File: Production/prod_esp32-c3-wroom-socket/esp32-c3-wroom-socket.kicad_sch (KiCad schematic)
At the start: 15 parts, among them J1 USB-C_Receptacle_Data_16P_GCT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, J3 USB-C_KUSBX-SL-CS1N14-B, SW2 SW_Push_SMD_6x3.5, U1 ESP32-C3-WROOM-02-N4, U2 AMS1117-3V3

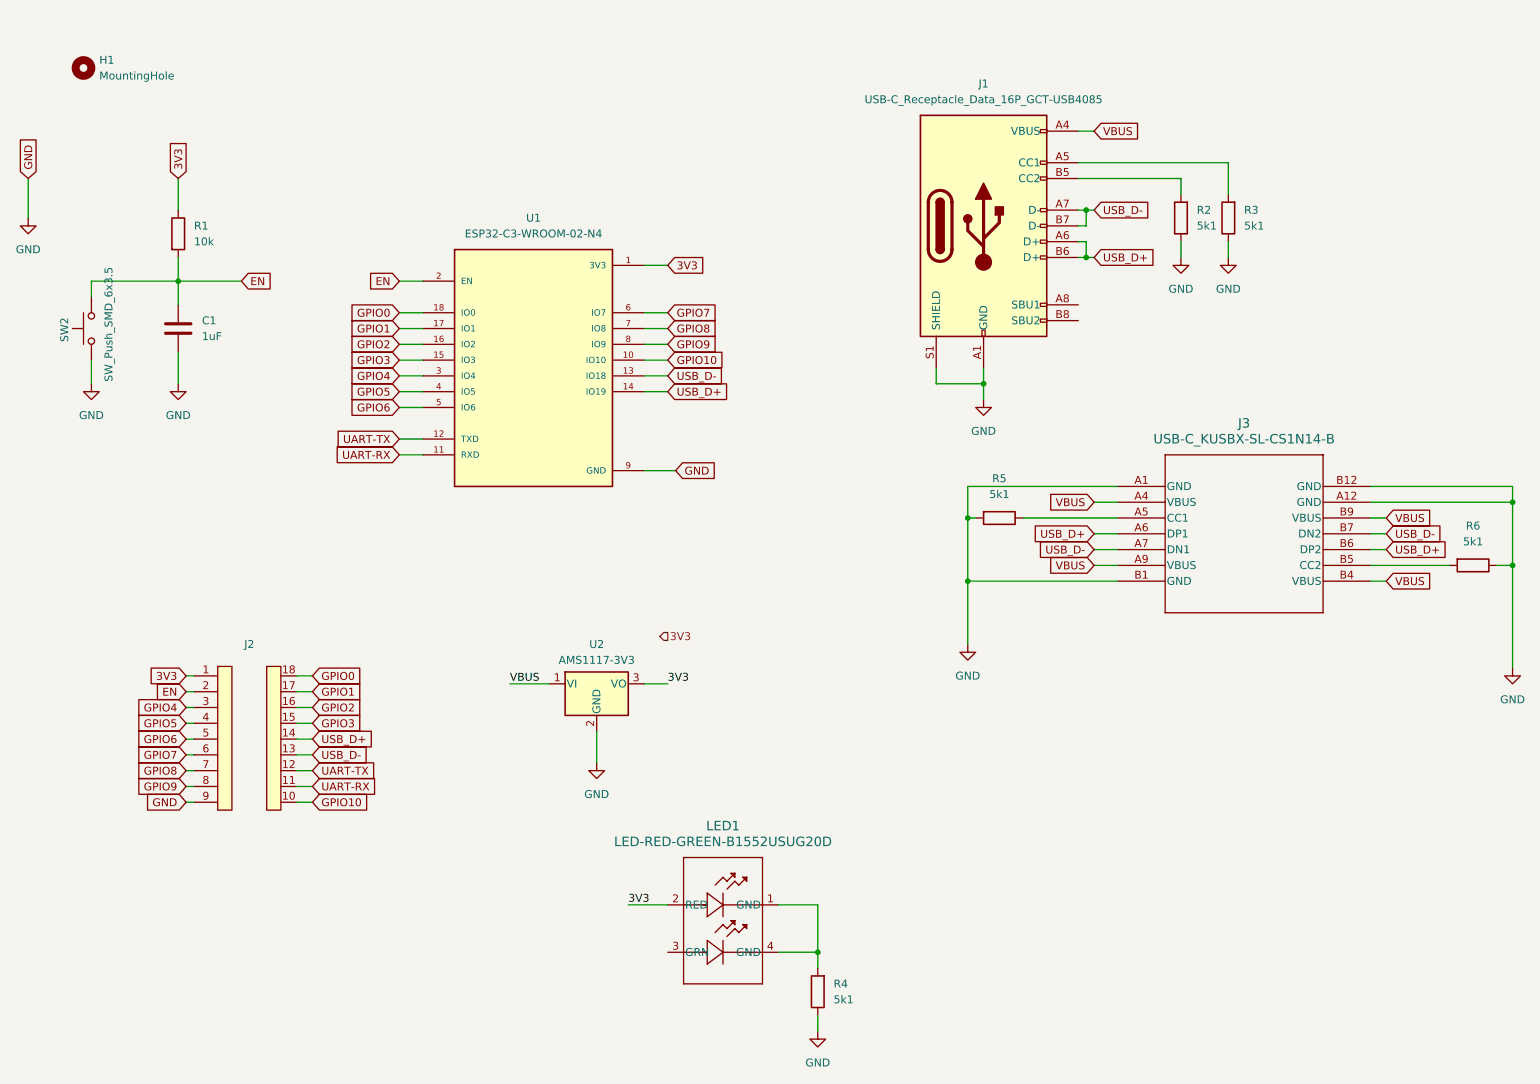
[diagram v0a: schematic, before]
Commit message: .
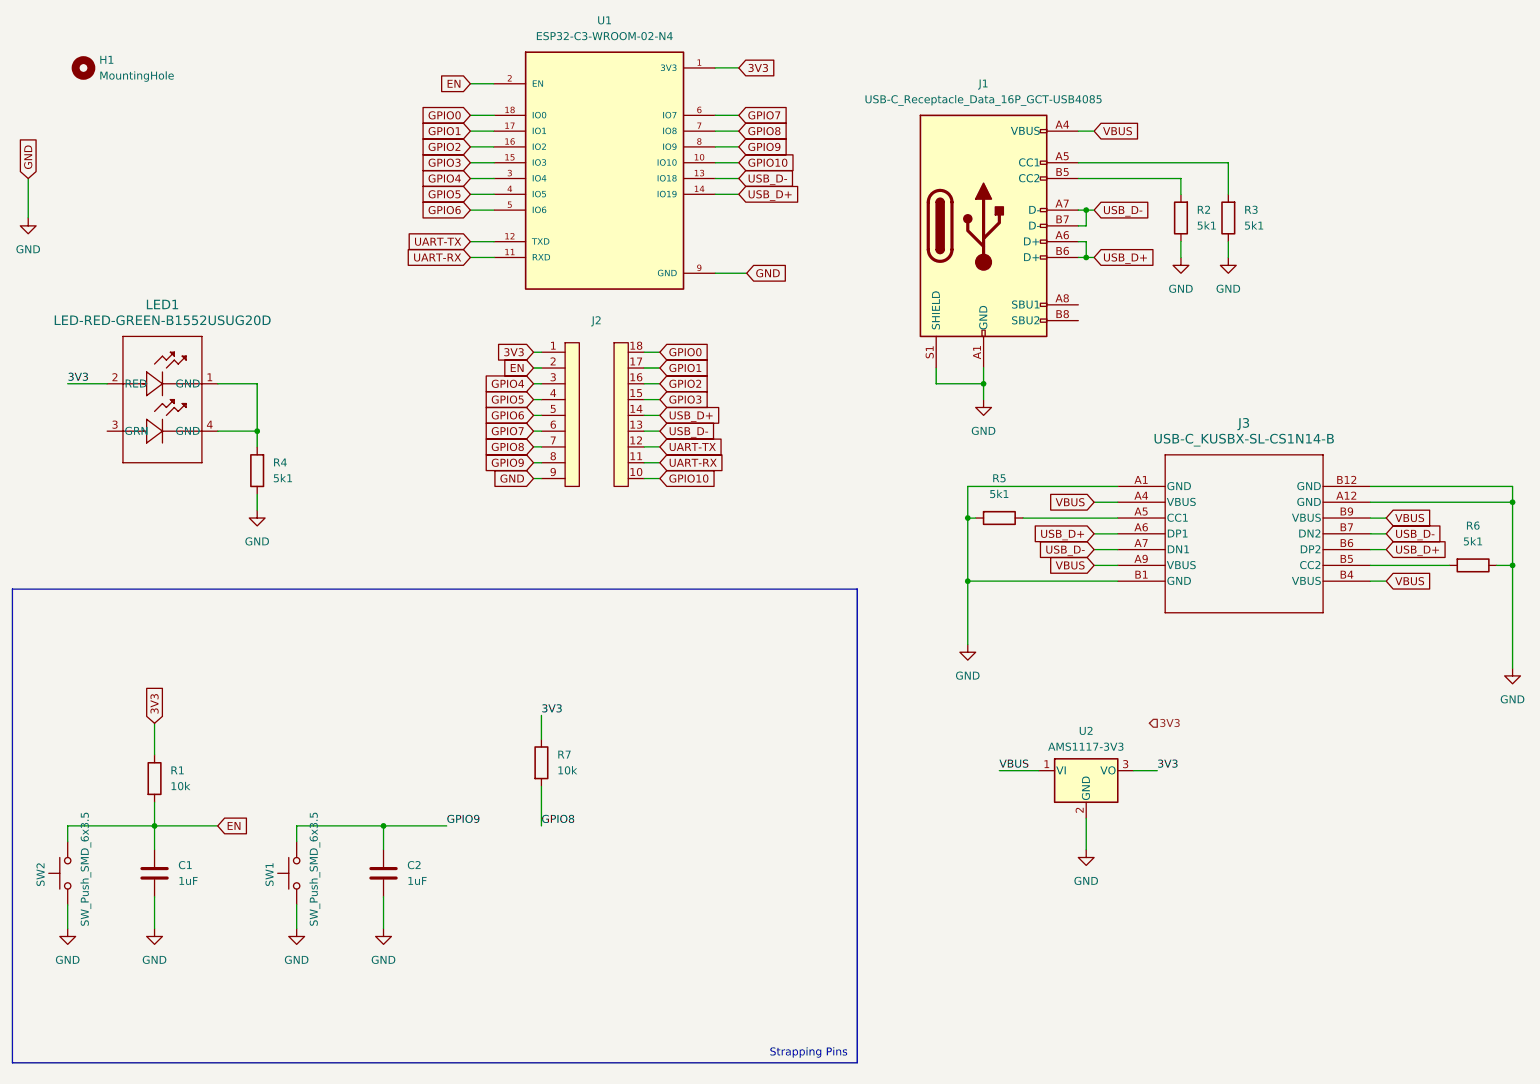
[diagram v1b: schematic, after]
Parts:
- added C2: 1uF, Resistor_SMD:R_0612_1632Metric_Pad1.18x3.40mm_HandSolder, symbol Device:C
- added R7: 10k, Resistor_SMD:R_1206_3216Metric_Pad1.30x1.75mm_HandSolder, symbol Device:R
- added SW1: SW_Push_SMD_6x3.5, Alexander Footprint Library:SW_PUSH_6x3.5mm, symbol Alexander_Library_Symbols:SW_Push_SMD_6x3.5
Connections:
- net 3V3: now also R7.1
- net GND: now also C2.2, SW1.1
- net GPIO8: now also R7.2
- net GPIO9: now also C2.1, SW1.2
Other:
- note added: "Strapping Pins"
- moved on the sheet: C1, J2, LED1, R1, R4, SW2, U1, U2
